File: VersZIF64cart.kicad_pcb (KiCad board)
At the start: 2 copper layers, 57.9 x 73.1 mm, 13 parts, among them J1 EXPANSION_PORT_C64, SW1 SW_DIP_x05, SW2 SW_Push, SW3 SW_Rotary2x3, U1 27512

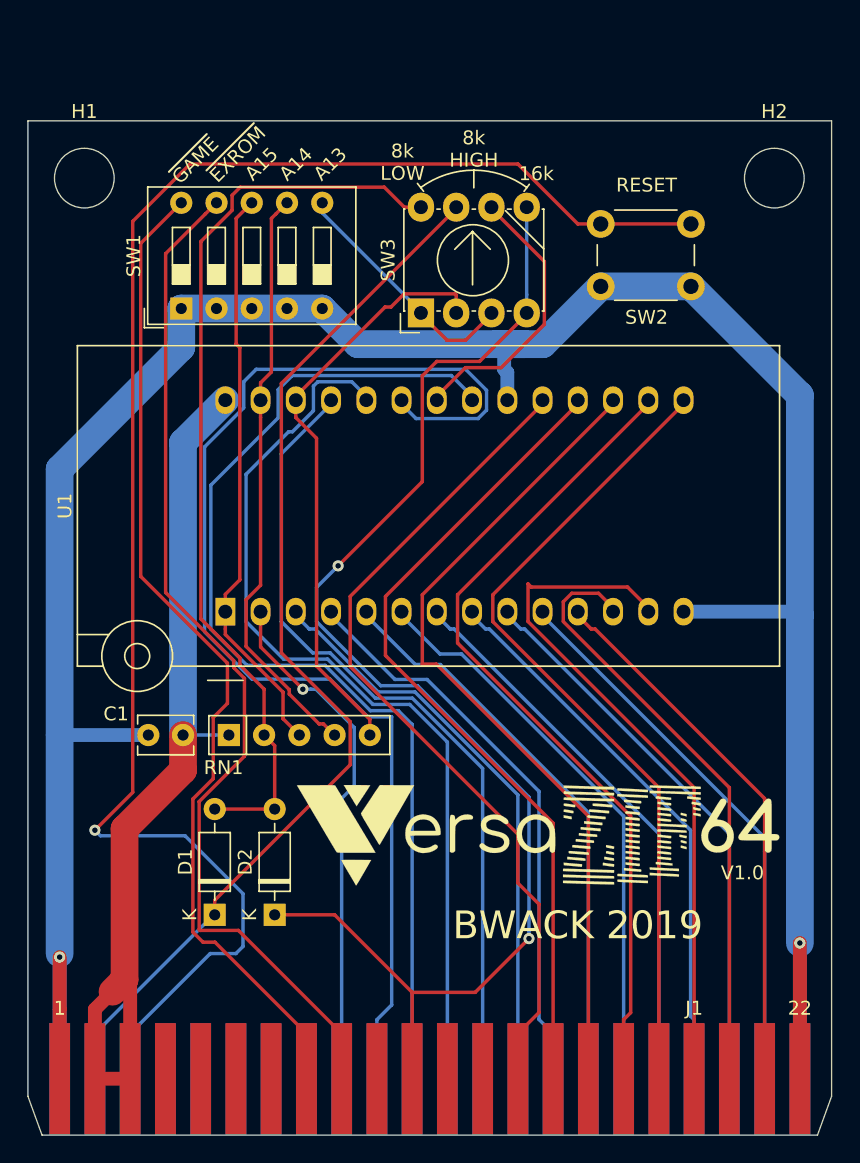
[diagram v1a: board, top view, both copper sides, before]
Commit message: V1.1
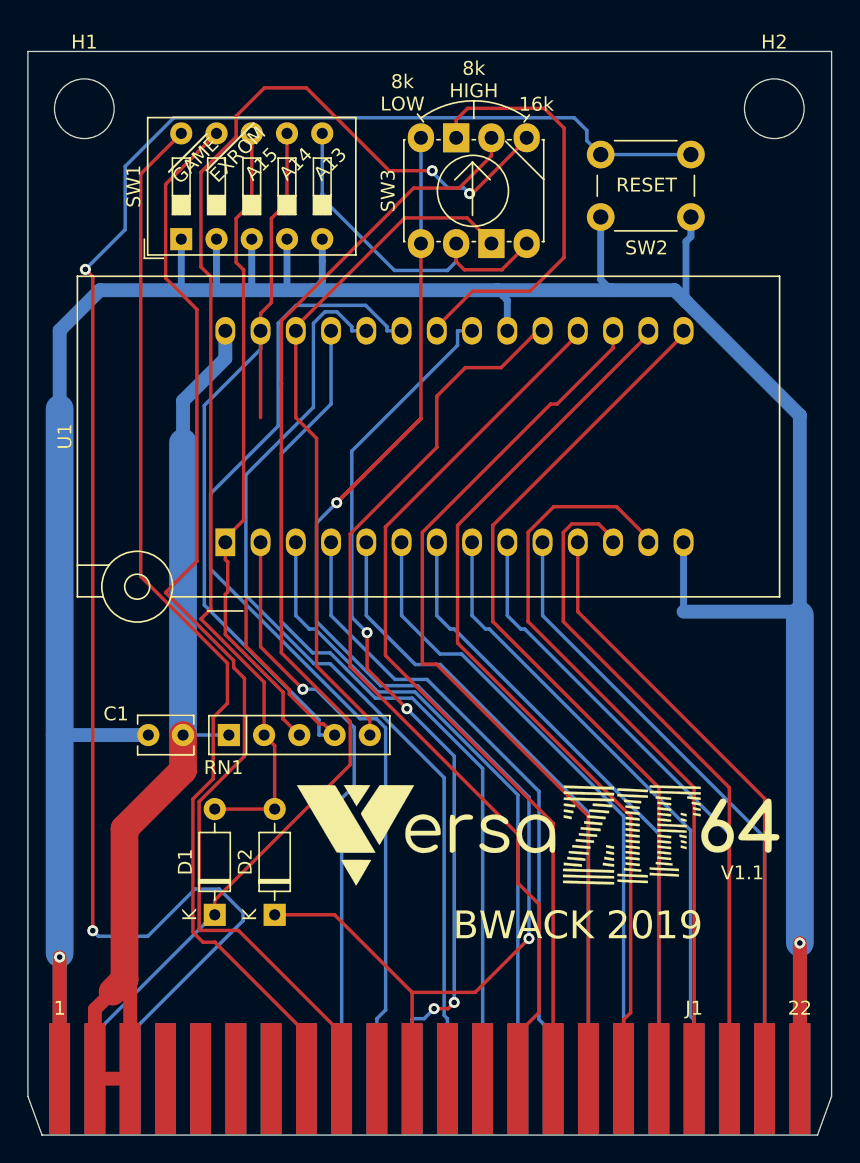
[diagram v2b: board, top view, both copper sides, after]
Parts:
- moved H1 5.00 mm to (27.2, 30.1)
- moved H2 5.00 mm to (76.9, 30.1)
- moved SW1 5.00 mm to (34.2, 39.5)
- moved SW2 5.00 mm to (64.4, 33.4)
- moved SW3 5.00 mm to (51.4, 39.8)
- moved U1 5.00 mm to (37.3, 61.3)
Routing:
- net GND: track 198.6 -> 234.0 mm
- net /DIP_A14: track 42.4 -> 69.2 mm
- net /~OEMIX~: track 66.1 -> 84.8 mm, vias 0 -> 2
- net /A11: track 88.7 -> 73.0 mm
- net /A10: track 77.4 -> 63.5 mm, vias 0 -> 4
- net /~ROM_OE~: track 20.2 -> 30.8 mm
- net Net-(J1-PadC): track 119.1 -> 128.7 mm, vias 1 -> 2
- net /~ROML~: track 97.1 -> 105.8 mm
- net /~ROMH~: track 77.7 -> 85.9 mm
- net /D7: track 60.9 -> 68.9 mm
- net /DIP_A13: track 17.7 -> 25.5 mm
- net /ROM_A13: track 42.6 -> 49.8 mm
- net /~EXROM~: track 74.2 -> 81.1 mm
- net /DIP_A15: track 41.6 -> 46.9 mm
- net /D5: track 60.1 -> 65.4 mm
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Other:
- board size 57.9 x 73.1 mm -> 57.9 x 78.1 mm
- board text added: "V1.1"
- board text removed: "V1.0"
